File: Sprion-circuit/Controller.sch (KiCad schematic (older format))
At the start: 1 part, among them U3 STM32F405RGTx

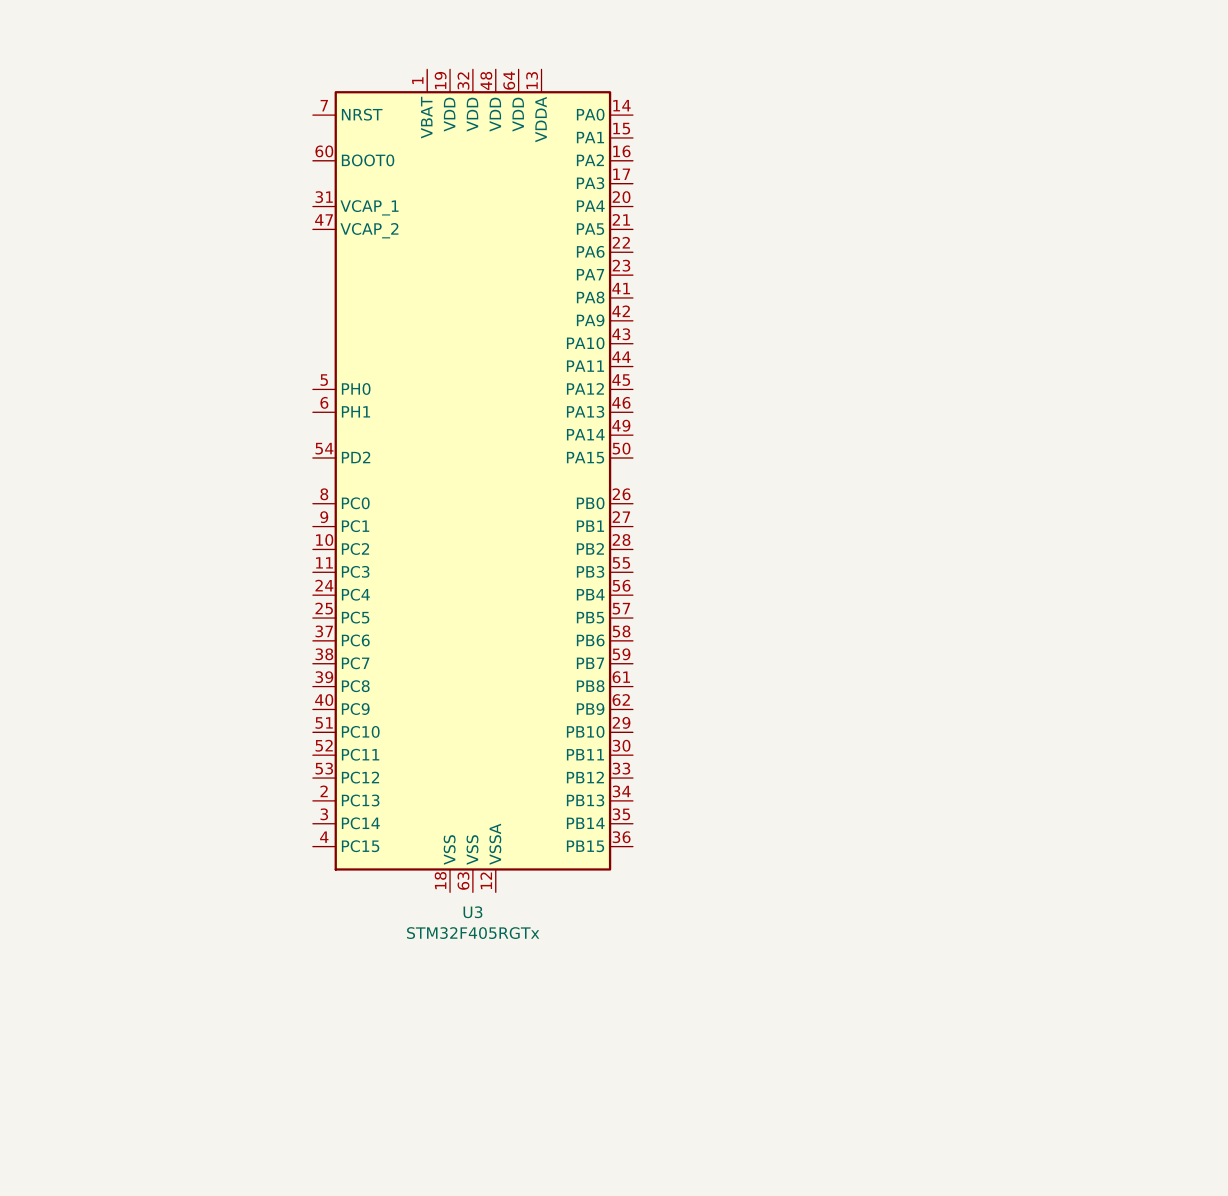
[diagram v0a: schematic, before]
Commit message: z
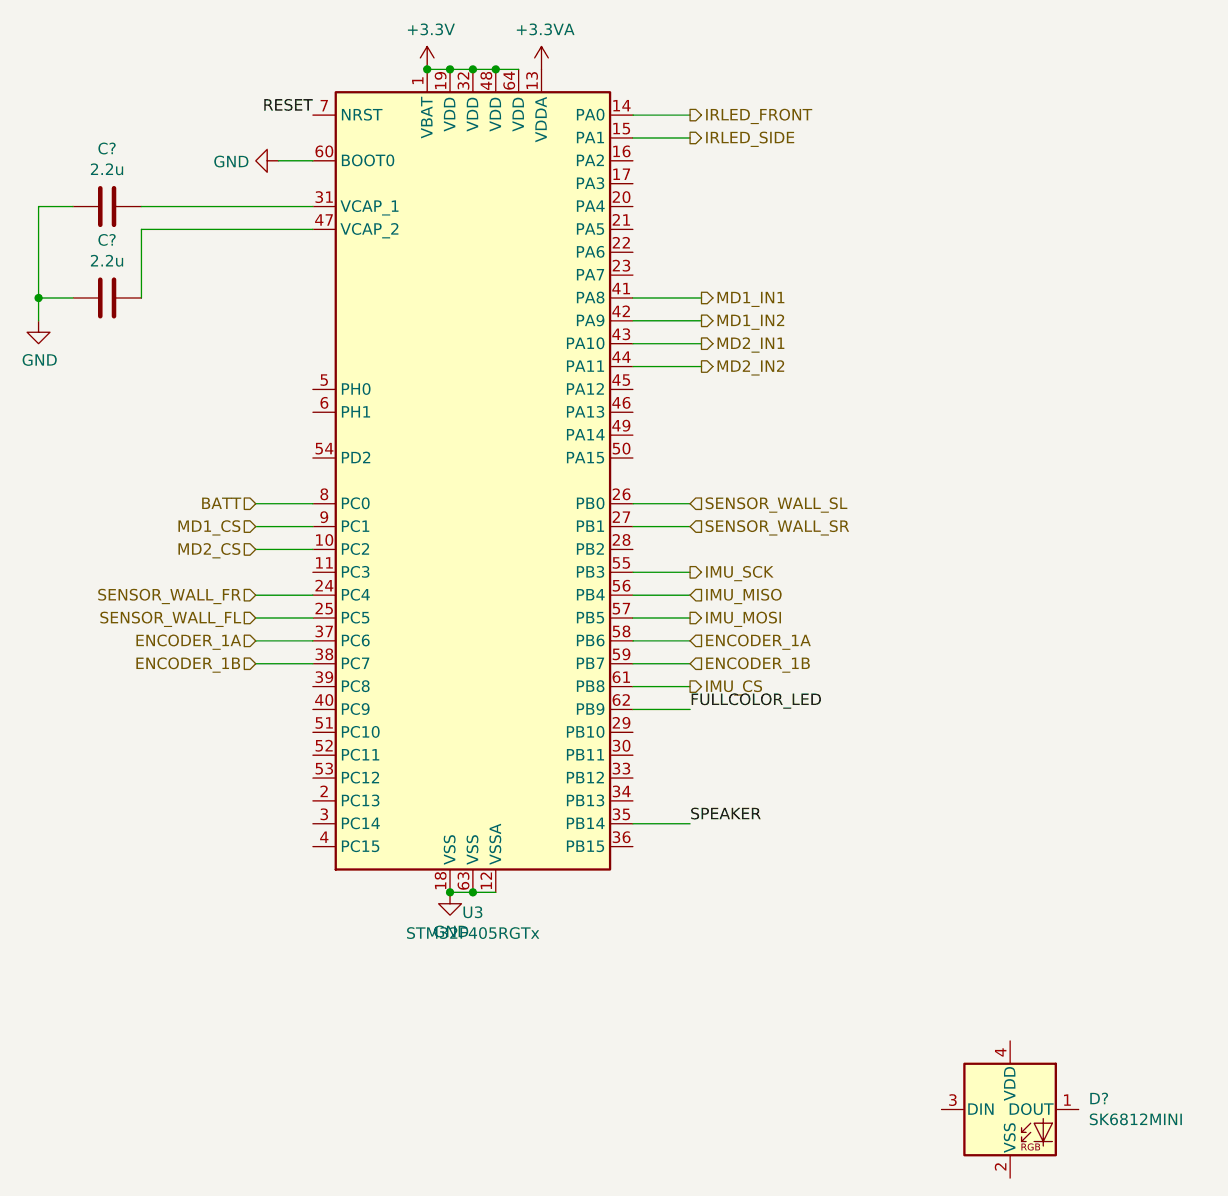
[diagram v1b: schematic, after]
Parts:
- added C? (x2): 2.2u, symbol Device:C
- added D?: SK6812MINI, LED_SMD:LED_SK6812MINI_PLCC4_3.5x3.5mm_P1.75mm, symbol LED:SK6812MINI
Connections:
- net +3V3: now reaches U3.1 (VBAT)
- net +3V3: now also U3.19 (VDD), U3.32 (VDD), U3.48 (VDD), U3.64 (VDD)
- net MD2_CS: now reaches U3.10 (PC2)
- net GND: now reaches U3.12 (VSSA)
- net GND: now also U3.18 (VSS), U3.60 (BOOT0), U3.63 (VSS), C?.2, C?.2
- net +3.3VA: now reaches U3.13 (VDDA)
- net IRLED_FRONT: now reaches U3.14 (PA0)
- net IRLED_SIDE: now reaches U3.15 (PA1)
- net SENSOR_WALL_FR: now reaches U3.24 (PC4)
- net SENSOR_WALL_FL: now reaches U3.25 (PC5)
- net SENSOR_WALL_SL: now reaches U3.26 (PB0)
- net SENSOR_WALL_SR: now reaches U3.27 (PB1)
- net at U3.31 (VCAP_1): now also C?.1
- net SPEAKER: now reaches U3.35 (PB14)
- net ENCODER_1A: now reaches U3.37 (PC6)
- net ENCODER_1A: now also U3.58 (PB6)
- net ENCODER_1B: now reaches U3.38 (PC7)
- net ENCODER_1B: now also U3.59 (PB7)
- net MD1_IN1: now reaches U3.41 (PA8)
- net MD1_IN2: now reaches U3.42 (PA9)
- net MD2_IN1: now reaches U3.43 (PA10)
- net MD2_IN2: now reaches U3.44 (PA11)
- net at U3.47 (VCAP_2): now also C?.1
- net IMU_SCK: now reaches U3.55 (PB3)
- net IMU_MISO: now reaches U3.56 (PB4)
- net IMU_MOSI: now reaches U3.57 (PB5)
- net IMU_CS: now reaches U3.61 (PB8)
- net FULLCOLOR_LED: now reaches U3.62 (PB9)
- net RESET: now reaches U3.7 (NRST)
- net BATT: now reaches U3.8 (PC0)
- net MD1_CS: now reaches U3.9 (PC1)
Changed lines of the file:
@@
 $Descr A4 11693 8268
 encoding utf-8
-Sheet 3 5
+Sheet 5 5
 Title ""
 Date ""
@@
 	1    0    0    -1
 $EndComp
+Wire Wire Line
+	3200 5300 3300 5300
+Connection ~ 3300 5300
+Wire Wire Line
+	3300 5300 3400 5300
+$Comp
+L power:GND #PWR?
+U 1 1 60EE0122
+P 3200 5300
+F 0 "#PWR?" H 3200 5050 50  0001 C CNN
+F 1 "GND" H 3205 5127 50  0000 C CNN
+F 2 "" H 3200 5300 50  0001 C CNN
+F 3 "" H 3200 5300 50  0001 C CNN
+	1    3200 5300
+	1    0    0    -1
+$EndComp
+Connection ~ 3200 5300
+$Comp
+L power:+3.3V #PWR?
+U 1 1 60EE1AE2
+P 3100 1700
+F 0 "#PWR?" H 3100 1550 50  0001 C CNN
+F 1 "+3.3V" H 3115 1873 50  0000 C CNN
+F 2 "" H 3100 1700 50  0001 C CNN
+F 3 "" H 3100 1700 50  0001 C CNN
+	1    3100 1700
+	1    0    0    -1
+$EndComp
+Wire Wire Line
+	3100 1700 3200 1700
+Connection ~ 3100 1700
+Connection ~ 3200 1700
+Wire Wire Line
+	3200 1700 3300 1700
+Connection ~ 3300 1700
+Wire Wire Line
+	3300 1700 3400 1700
+Connection ~ 3400 1700
+Wire Wire Line
+	3400 1700 3500 1700
+$Comp
+L power:+3.3VA #PWR?
+U 1 1 60EE2B83
+P 3600 1700
+F 0 "#PWR?" H 3600 1550 50  0001 C CNN
+F 1 "+3.3VA" H 3615 1873 50  0000 C CNN
+F 2 "" H 3600 1700 50  0001 C CNN
+F 3 "" H 3600 1700 50  0001 C CNN
+	1    3600 1700
+	1    0    0    -1
+$EndComp
+Text Label 2600 1900 2    50   ~ 0
+RESET
+$Comp
+L power:GND #PWR?
+U 1 1 60EE357E
+P 2450 2100
+F 0 "#PWR?" H 2450 1850 50  0001 C CNN
+F 1 "GND" V 2455 1972 50  0000 R CNN
+F 2 "" H 2450 2100 50  0001 C CNN
+F 3 "" H 2450 2100 50  0001 C CNN
+	1    2450 2100
+	0    1    1    0
+$EndComp
+Wire Wire Line
+	2450 2100 2600 2100
+Text HLabel 4250 3900 2    50   Output ~ 0
+IMU_SCK
+Text HLabel 4250 4000 2    50   Input ~ 0
+IMU_MISO
+Text HLabel 4250 4100 2    50   Output ~ 0
+IMU_MOSI
+Wire Wire Line
+	4250 3900 4000 3900
+Wire Wire Line
+	4250 4000 4000 4000
+Wire Wire Line
+	4250 4100 4000 4100
+Text HLabel 2350 4300 0    50   Input ~ 0
+ENCODER_1B
+Text HLabel 2350 4200 0    50   Input ~ 0
+ENCODER_1A
+Text HLabel 4250 4400 2    50   Output ~ 0
+IMU_CS
+Wire Wire Line
+	4250 4400 4000 4400
+Wire Wire Line
+	2350 4300 2600 4300
+Wire Wire Line
+	2350 4200 2600 4200
+Text HLabel 4250 4200 2    50   Input ~ 0
+ENCODER_1A
+Text HLabel 4250 4300 2    50   Input ~ 0
+ENCODER_1B
+Wire Wire Line
+	4250 4200 4000 4200
+Wire Wire Line
+	4250 4300 4000 4300
+Text HLabel 2350 3600 0    50   Input ~ 0
+BATT
+Wire Wire Line
+	2600 3600 2350 3600
+Text HLabel 4250 1900 2    50   Output ~ 0
+IRLED_FRONT
+Text HLabel 4250 2000 2    50   Output ~ 0
+IRLED_SIDE
+Wire Wire Line
+	4000 1900 4250 1900
+Wire Wire Line
+	4000 2000 4250 2000
+Text HLabel 4300 2700 2    50   Output ~ 0
+MD1_IN1
+Text HLabel 4300 2800 2    50   Output ~ 0
+MD1_IN2
+Text HLabel 4300 2900 2    50   Output ~ 0
+MD2_IN1
+Text HLabel 4300 3000 2    50   Output ~ 0
+MD2_IN2
+Wire Wire Line
+	4000 2700 4300 2700
+Wire Wire Line
+	4000 2800 4300 2800
+Wire Wire Line
+	4000 2900 4300 2900
+Wire Wire Line
+	4000 3000 4300 3000
+Text HLabel 2350 3700 0    50   Input ~ 0
+MD1_CS
+Text HLabel 2350 3800 0    50   Input ~ 0
+MD2_CS
+Wire Wire Line
+	2350 3700 2600 3700
+Wire Wire Line
+	2350 3800 2600 3800
+Text HLabel 2350 4000 0    50   Input ~ 0
+SENSOR_WALL_FR
+Text HLabel 2350 4100 0    50   Input ~ 0
+SENSOR_WALL_FL
+Text HLabel 4250 3700 2    50   Input ~ 0
+SENSOR_WALL_SR
+Text HLabel 4250 3600 2    50   Input ~ 0
+SENSOR_WALL_SL
+Wire Wire Line
+	4000 3600 4250 3600
+Wire Wire Line
+	4000 3700 4250 3700
+$Comp
+L Device:C C?
+U 1 1 60EF0F88
+P 1700 2300
+F 0 "C?" V 1448 2300 50  0000 C CNN
+F 1 "2.2u" V 1539 2300 50  0000 C CNN
+F 2 "" H 1738 2150 50  0001 C CNN
+F 3 "~" H 1700 2300 50  0001 C CNN
+	1    1700 2300
+	0    1    1    0
+$EndComp
+$Comp
+L Device:C C?
+U 1 1 60EF1ACA
+P 1700 2700
+F 0 "C?" V 1448 2700 50  0000 C CNN
+F 1 "2.2u" V 1539 2700 50  0000 C CNN
+F 2 "" H 1738 2550 50  0001 C CNN
+F 3 "~" H 1700 2700 50  0001 C CNN
+	1    1700 2700
+	0    1    1    0
+$EndComp
+Wire Wire Line
+	1850 2300 2600 2300
+Wire Wire Line
+	2600 2400 1850 2400
+Wire Wire Line
+	1850 2400 1850 2700
+$Comp
+L power:GND #PWR?
+U 1 1 60EF339E
+P 1400 2800
+F 0 "#PWR?" H 1400 2550 50  0001 C CNN
+F 1 "GND" H 1405 2627 50  0000 C CNN
+F 2 "" H 1400 2800 50  0001 C CNN
+F 3 "" H 1400 2800 50  0001 C CNN
+	1    1400 2800
+	1    0    0    -1
+$EndComp
+Wire Wire Line
+	1550 2700 1400 2700
+Wire Wire Line
+	1400 2700 1400 2800
+Wire Wire Line
+	1550 2300 1400 2300
+Wire Wire Line
+	1400 2300 1400 2700
+Connection ~ 1400 2700
+$Comp
+L LED:SK6812MINI D?
+U 1 1 60EFAFD7
+P 5650 6250
+F 0 "D?" H 5994 6296 50  0000 L CNN
+F 1 "SK6812MINI" H 5994 6205 50  0000 L CNN
+F 2 "LED_SMD:LED_SK6812MINI_PLCC4_3.5x3.5mm_P1.75mm" H 5700 5950 50  0001 L TNN
+F 3 "https://cdn-shop.adafruit.com/product-files/2686/SK6812MINI_REV.01-1-2.pdf" H 5750 5875 50  0001 L TNN
+	1    5650 6250
+	1    0    0    -1
+$EndComp
+Wire Wire Line
+	2350 4000 2600 4000
+Wire Wire Line
+	2350 4100 2600 4100
+Text Label 4250 5000 0    50   ~ 0
+SPEAKER
+Text Label 4250 4500 0    50   ~ 0
+FULLCOLOR_LED
+Wire Wire Line
+	4000 4500 4250 4500
+Wire Wire Line
+	4000 5000 4250 5000
 $EndSCHEMATC

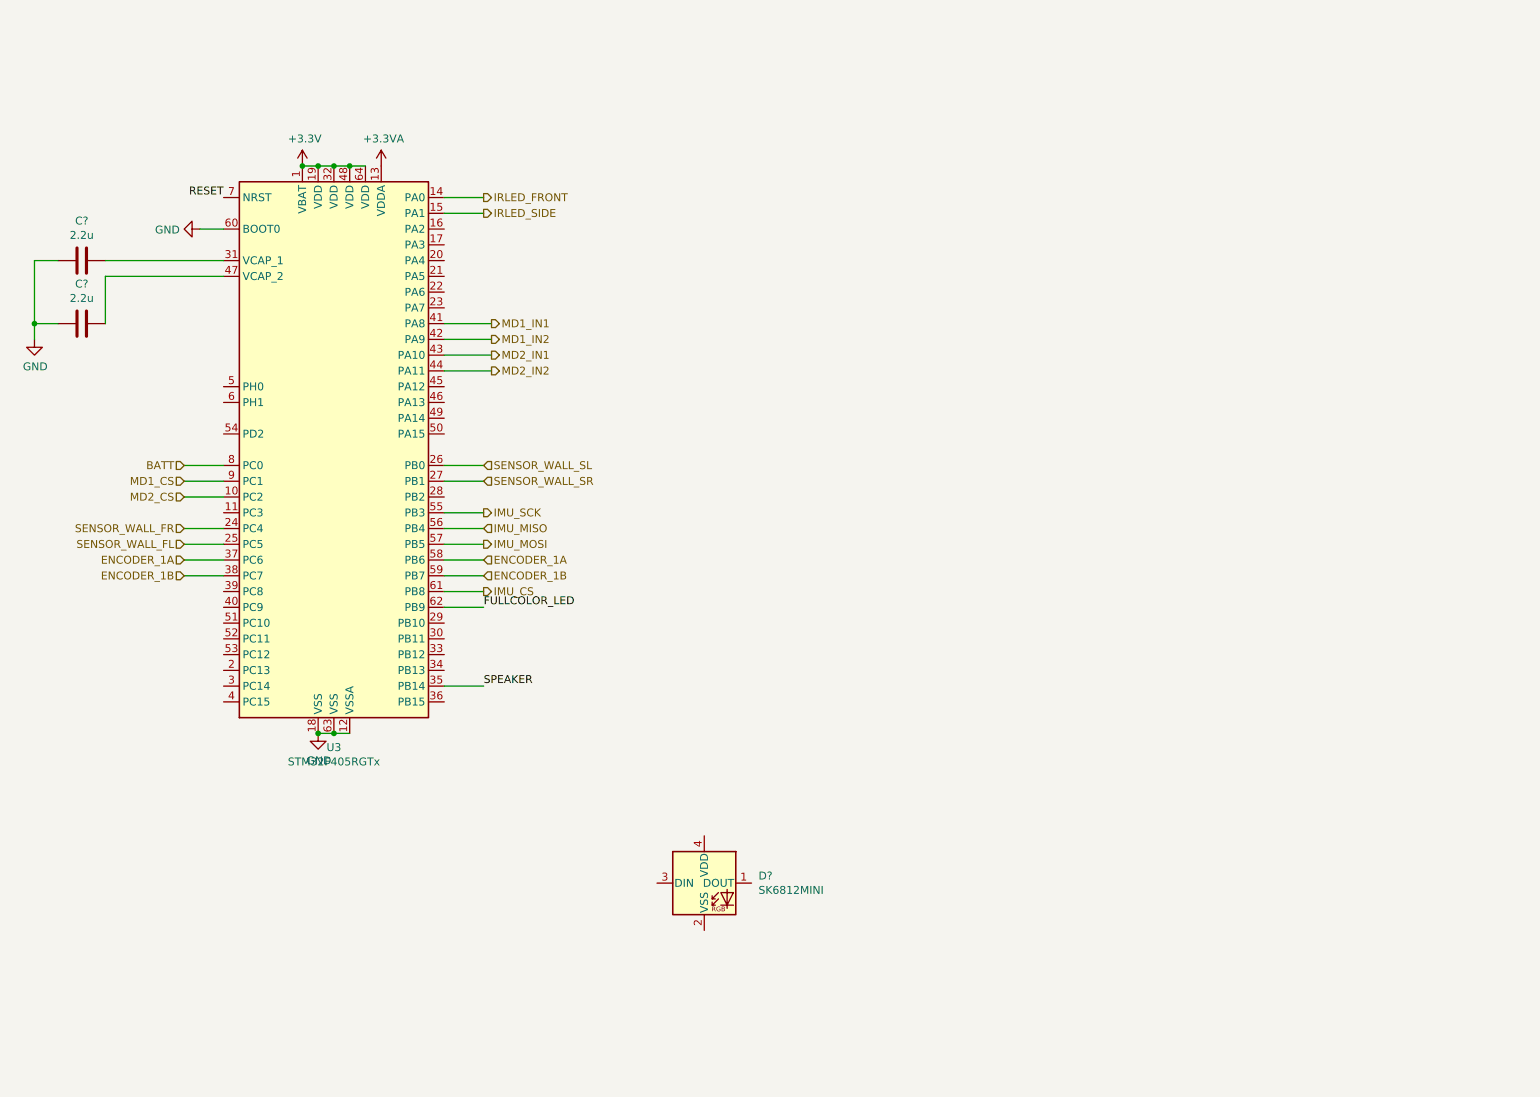
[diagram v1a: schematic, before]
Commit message: :fix　いろいろ
後で書きます
とりあえず寝ます
許してください
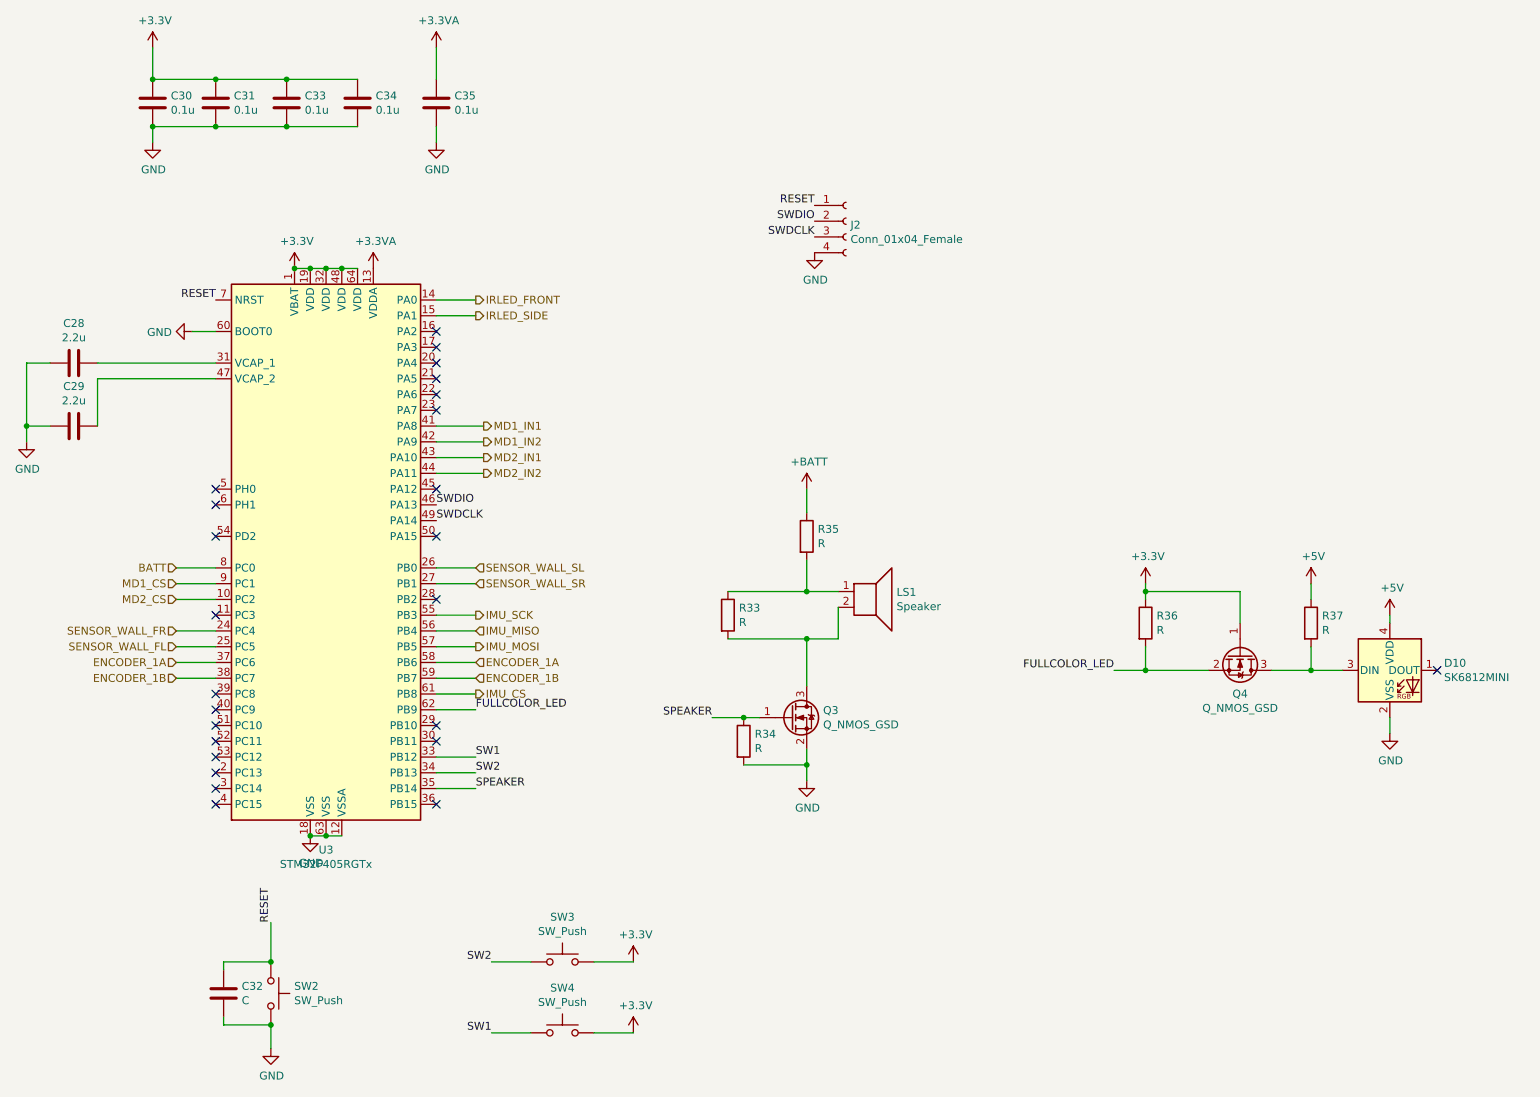
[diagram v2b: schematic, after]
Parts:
- added C30, C31, C33, C34, C35: 0.1u, symbol Device:C
- added C32: C, symbol Device:C
- added J2: Conn_01x04_Female, symbol Connector:Conn_01x04_Female
- added LS1: Speaker, symbol Device:Speaker
- added Q3, Q4: Q_NMOS_GSD, symbol Device:Q_NMOS_GSD
- added R33, R34, R35, R36, R37: R, symbol Device:R
- added SW2, SW3, SW4: SW_Push, symbol Switch:SW_Push
- gave numbers to parts that had none: 3
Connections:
- net +3.3VA: now also C35.1
- net +3V3: now also C30.1, C31.1, C33.1, C34.1, Q4.1 (G), R36.1, SW3.2, SW4.2
- net FULLCOLOR_LED: now also Q4.2 (S), R36.2
- net GND: now also D10.2 (VSS), C30.2, C31.2, C32.2, C33.2, C34.2, C35.2, J2.4 (Pin_4), Q3.2 (S), R34.2, SW2.2
- net RESET: now also C32.1, J2.1 (Pin_1), SW2.1
- net SPEAKER: now also Q3.1 (G), R34.1
- net at D10.3 (DIN): now also Q4.3 (D), R37.2
- net +5V: now reaches D10.4 (VDD)
- net +5V: now also R37.1
- net SW1: now reaches U3.33 (PB12)
- net SW1: now also SW4.1
- net SW2: now reaches U3.34 (PB13)
- net SW2: now also SW3.1
- net SWDIO: now reaches U3.46 (PA13)
- net SWDIO: now also J2.2 (Pin_2)
- net SWDCLK: now reaches U3.49 (PA14)
- net SWDCLK: now also J2.3 (Pin_3)
- new net: LS1.1, R33.1, R35.2
- new net: LS1.2, Q3.3 (D), R33.2
- new net +BATT: R35.1
- no-connect marks 0 -> 25
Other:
- moved on the sheet: C28, C29, D10, U3
